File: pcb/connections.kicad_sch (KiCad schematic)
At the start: 5 parts, among them J201 Conn_01x20_Female, J202 Conn_01x20_Female, J203 Conn_01x20_Female, J204 Conn_01x20_Female, J205 Conn_01x20_Female

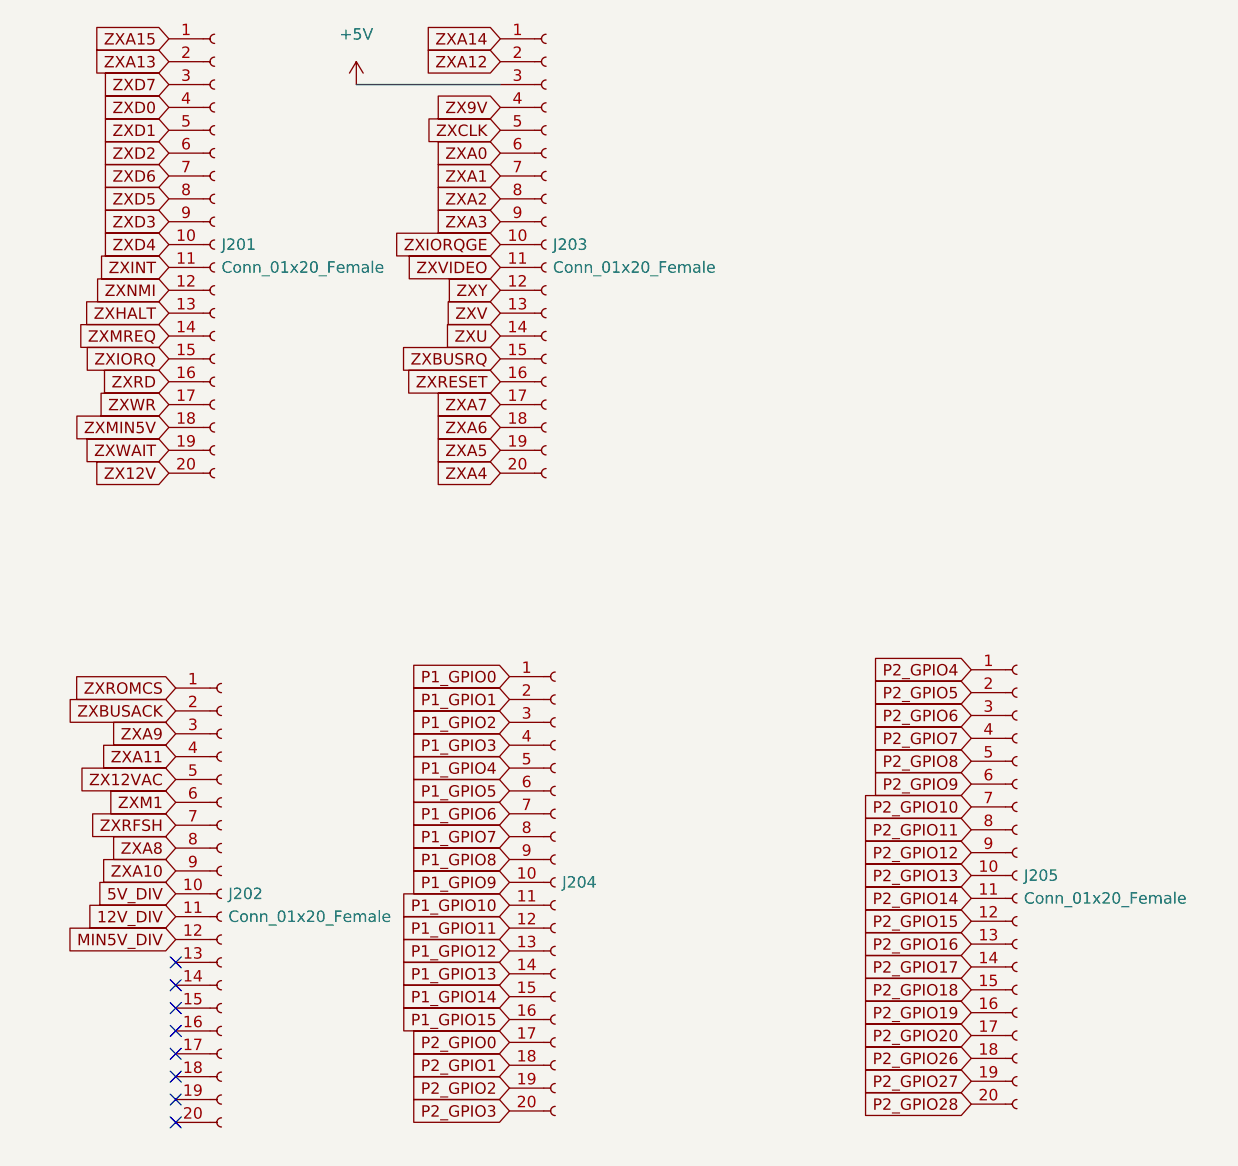
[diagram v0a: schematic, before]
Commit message: schematic reworked, it's time to relayout the board. checkpoint here
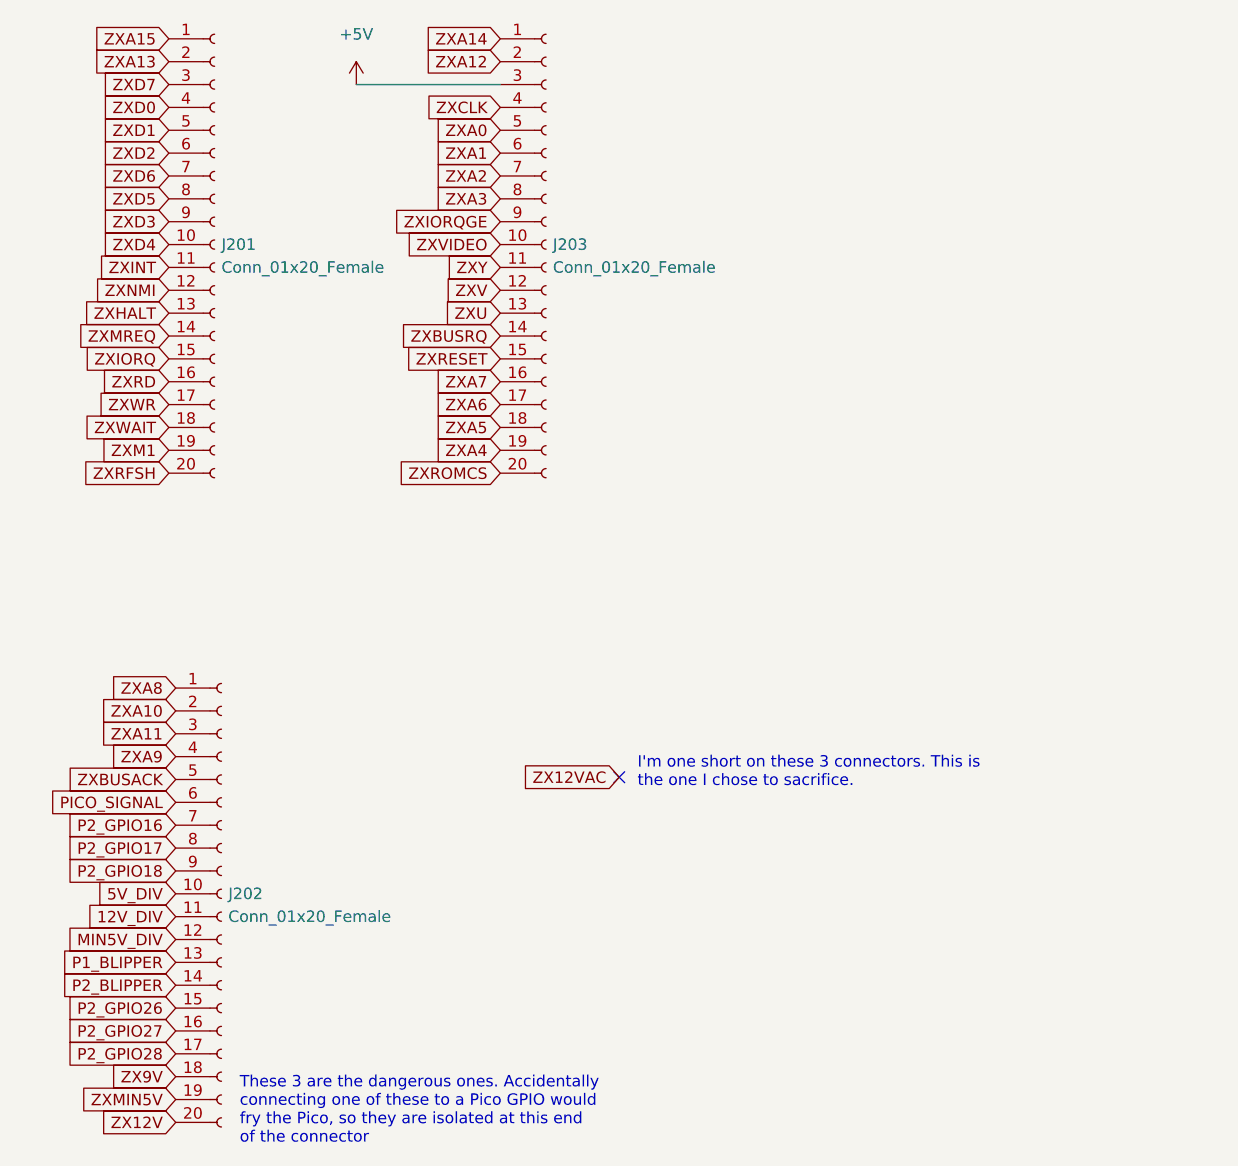
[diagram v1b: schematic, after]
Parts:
- removed J204, J205: Conn_01x20_Female, Connector_PinSocket_2.54mm:PinSocket_1x20_P2.54mm_Vertical, symbol Connector:Conn_01x20_Female
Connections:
- net P2_GPIO16: now also J202.7 (Pin_7)
- net P2_GPIO17: now also J202.8 (Pin_8)
- net P2_GPIO18: now also J202.9 (Pin_9)
- net P2_GPIO26: now also J202.15 (Pin_15)
- net P2_GPIO27: now also J202.16 (Pin_16)
- net P2_GPIO28: now also J202.17 (Pin_17)
- net ZX12V: now also J202.20 (Pin_20); no longer J201.20 (Pin_20)
- net ZX12VAC: no longer J202.5 (Pin_5)
- net ZX9V: now also J202.18 (Pin_18); no longer J203.4 (Pin_4)
- net ZXA0: now also J203.5 (Pin_5); no longer J203.6 (Pin_6)
- net ZXA1: now also J203.6 (Pin_6); no longer J203.7 (Pin_7)
- net ZXA10: now also J202.2 (Pin_2); no longer J202.9 (Pin_9)
- net ZXA11: now also J202.3 (Pin_3); no longer J202.4 (Pin_4)
- net ZXA2: now also J203.7 (Pin_7); no longer J203.8 (Pin_8)
- net ZXA3: now also J203.8 (Pin_8); no longer J203.9 (Pin_9)
- net ZXA4: now also J203.19 (Pin_19); no longer J203.20 (Pin_20)
- net ZXA5: now also J203.18 (Pin_18); no longer J203.19 (Pin_19)
- net ZXA6: now also J203.17 (Pin_17); no longer J203.18 (Pin_18)
- net ZXA7: now also J203.16 (Pin_16); no longer J203.17 (Pin_17)
- net ZXA8: now also J202.1 (Pin_1); no longer J202.8 (Pin_8)
- net ZXA9: now also J202.4 (Pin_4); no longer J202.3 (Pin_3)
- net ZXBUSACK: now also J202.5 (Pin_5); no longer J202.2 (Pin_2)
- net ZXBUSRQ: now also J203.14 (Pin_14); no longer J203.15 (Pin_15)
- net ZXCLK: now also J203.4 (Pin_4); no longer J203.5 (Pin_5)
- net ZXIORQGE: now also J203.9 (Pin_9); no longer J203.10 (Pin_10)
- net ZXM1: now also J201.19 (Pin_19); no longer J202.6 (Pin_6)
- net ZXMIN5V: now also J202.19 (Pin_19); no longer J201.18 (Pin_18)
- net ZXRESET: now also J203.15 (Pin_15); no longer J203.16 (Pin_16)
- net ZXRFSH: now also J201.20 (Pin_20); no longer J202.7 (Pin_7)
- net ZXROMCS: now also J203.20 (Pin_20); no longer J202.1 (Pin_1)
- net ZXU: now also J203.13 (Pin_13); no longer J203.14 (Pin_14)
- net ZXV: now also J203.12 (Pin_12); no longer J203.13 (Pin_13)
- net ZXVIDEO: now also J203.10 (Pin_10); no longer J203.11 (Pin_11)
- net ZXWAIT: now also J201.18 (Pin_18); no longer J201.19 (Pin_19)
- net ZXY: now also J203.11 (Pin_11); no longer J203.12 (Pin_12)
- net P1_BLIPPER: now reaches J202.13 (Pin_13)
- net P2_BLIPPER: now reaches J202.14 (Pin_14)
- new net PICO_SIGNAL: J202.6 (Pin_6)
- no-connect marks 8 -> 1
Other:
- note added: "I'm one short on these 3 connectors. This is the one I chose to sacrifice."
- note added: "These 3 are the dangerous ones. Accidentally connecting one of these to a Pico GPIO would fry the Pico, so they are isolated at this end of the connector"
